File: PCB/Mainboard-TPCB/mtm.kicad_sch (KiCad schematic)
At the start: 3 parts, among them J10 MTM-USBStem, J12 PinHeader 02x04, J9 PinHeader 01x03

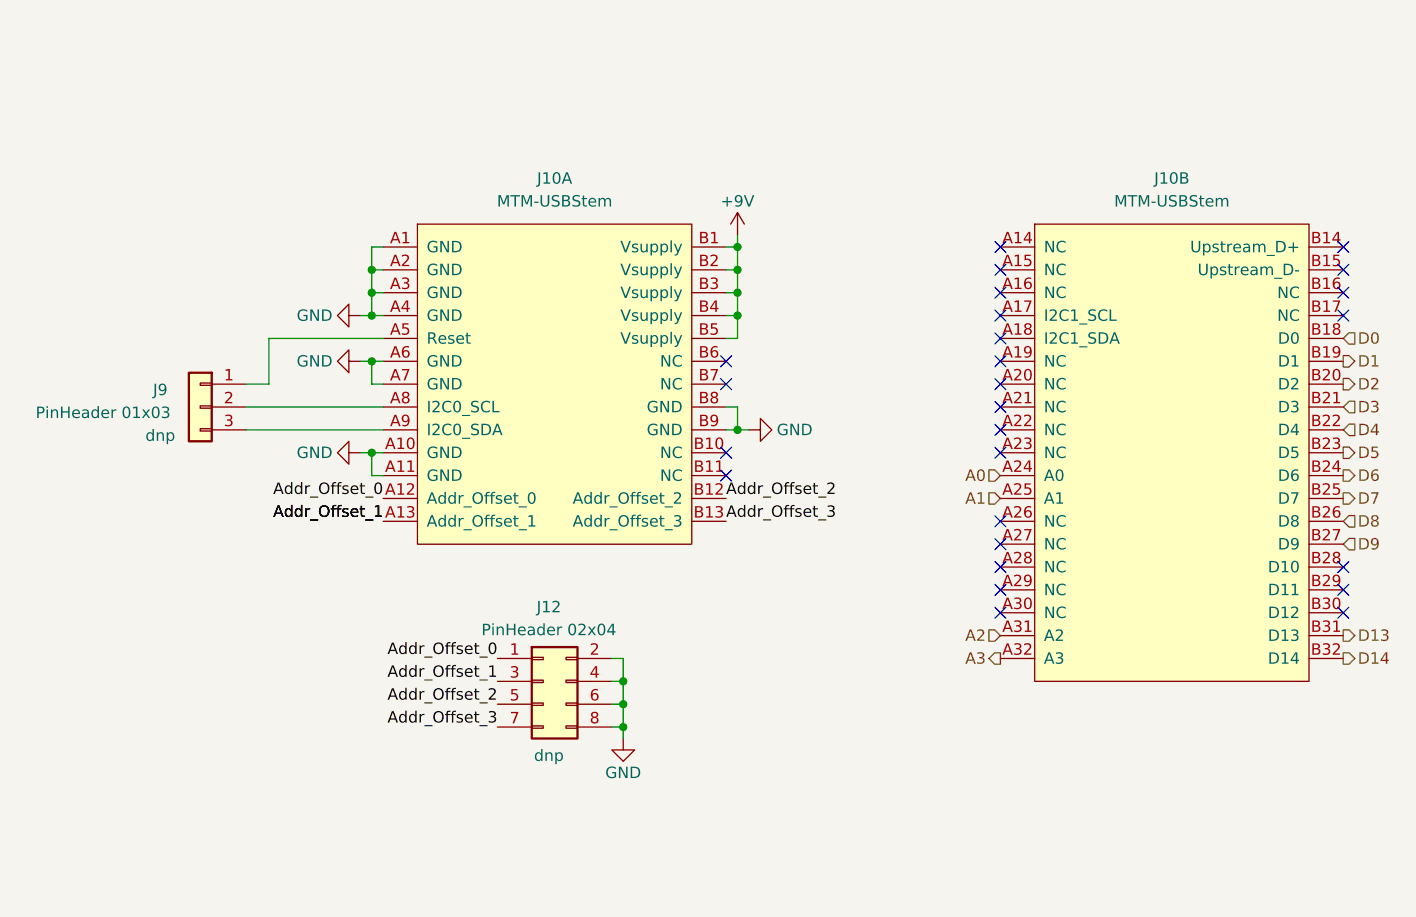
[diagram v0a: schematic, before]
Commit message: TPCB files V2
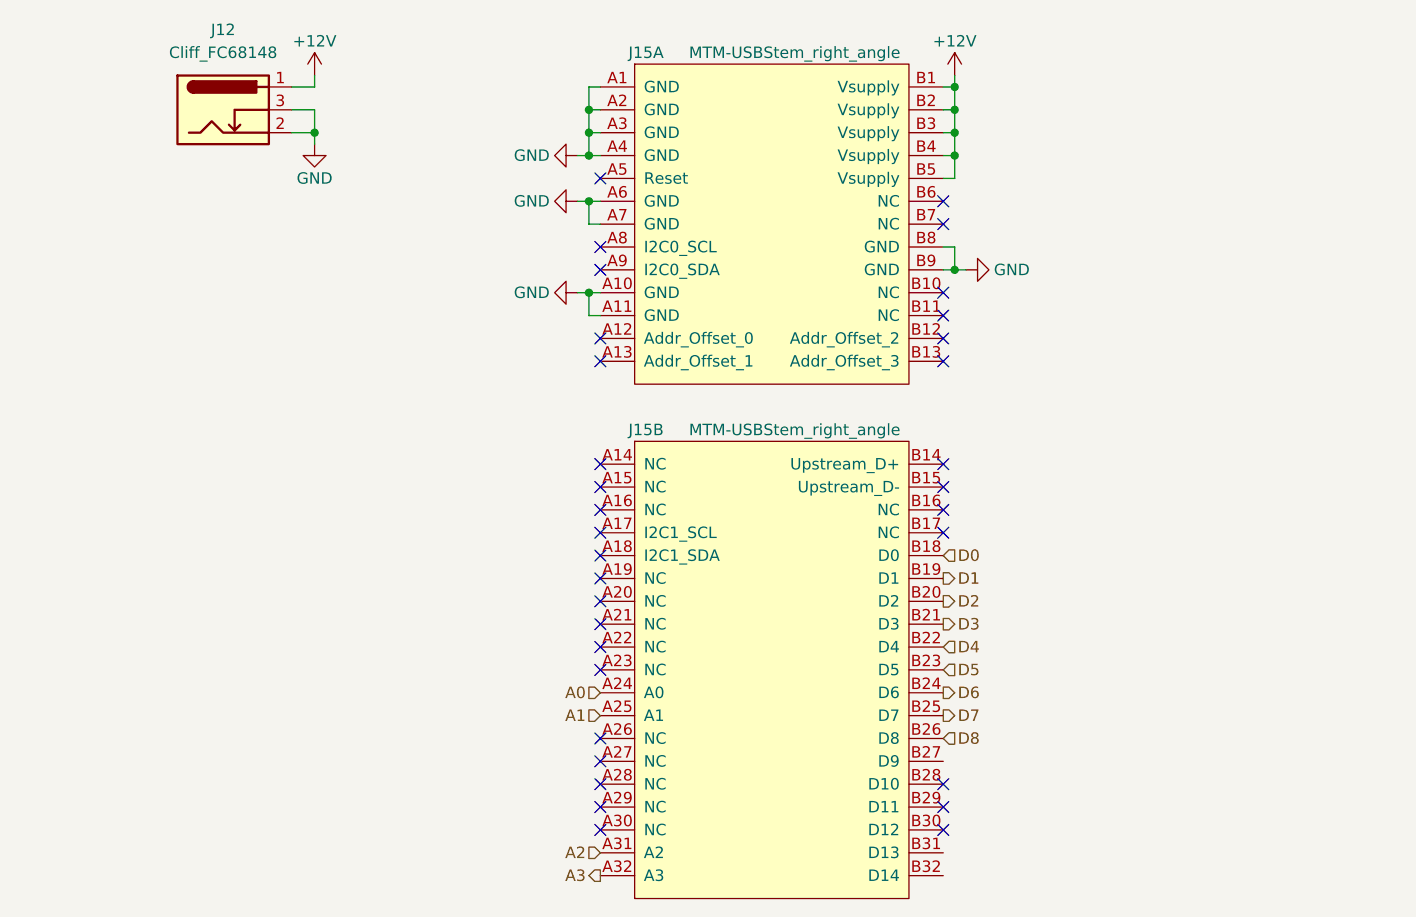
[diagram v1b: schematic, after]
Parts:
- removed J10: MTM-USBStem, zoudio_footprints:Amphenol_10018784-10201TLF, symbol zoudio_symbols:MTM-USBStem
- removed J12: PinHeader 02x04, Connector_PinHeader_2.54mm:PinHeader_2x04_P2.54mm_Vertical, symbol Connector_Generic:Conn_02x04_Odd_Even
- removed J9: PinHeader 01x03, Connector_PinHeader_2.54mm:PinHeader_1x03_P2.54mm_Vertical, symbol Connector_Generic:Conn_01x03
- added J12: Cliff_FC68148, zoudio_footprints:FC68148, symbol zoudio_symbols:Cliff_FC68148
- added J15: MTM-USBStem_right_angle, zoudio_footprints:SAMTEC_PCIE-064-02-X-D-RA, symbol zoudio_symbols:MTM-USBStem_right_angle
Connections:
- net A0: now also J15.A24 (A0)
- net A1: now also J15.A25 (A1)
- net A2: now also J15.A31 (A2)
- net A3: now also J15.A32 (A3)
- net D0: now also J15.B18 (D0)
- net D1: now also J15.B19 (D1)
- net D2: now also J15.B20 (D2)
- net D3: now also J15.B21 (D3)
- net D4: now also J15.B22 (D4)
- net D5: now also J15.B23 (D5)
- net D6: now also J15.B24 (D6)
- net D7: now also J15.B25 (D7)
- net D8: now also J15.B26 (D8)
- net GND: now also J12.2, J12.3, J15.A1 (GND), J15.A10 (GND), J15.A11 (GND), J15.A2 (GND), J15.A3 (GND), J15.A4 (GND), J15.A6 (GND), J15.A7 (GND), J15.B8 (GND), J15.B9 (GND)
- new net +12V: J12.1, J15.B1 (Vsupply), J15.B2 (Vsupply), J15.B3 (Vsupply), J15.B4 (Vsupply), J15.B5 (Vsupply)
- no-connect marks 26 -> 33
